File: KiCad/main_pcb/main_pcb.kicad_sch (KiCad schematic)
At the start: 14 parts, among them U5 TI TXB0104DR, U7 TI TXB0104DR, U8 CH340C

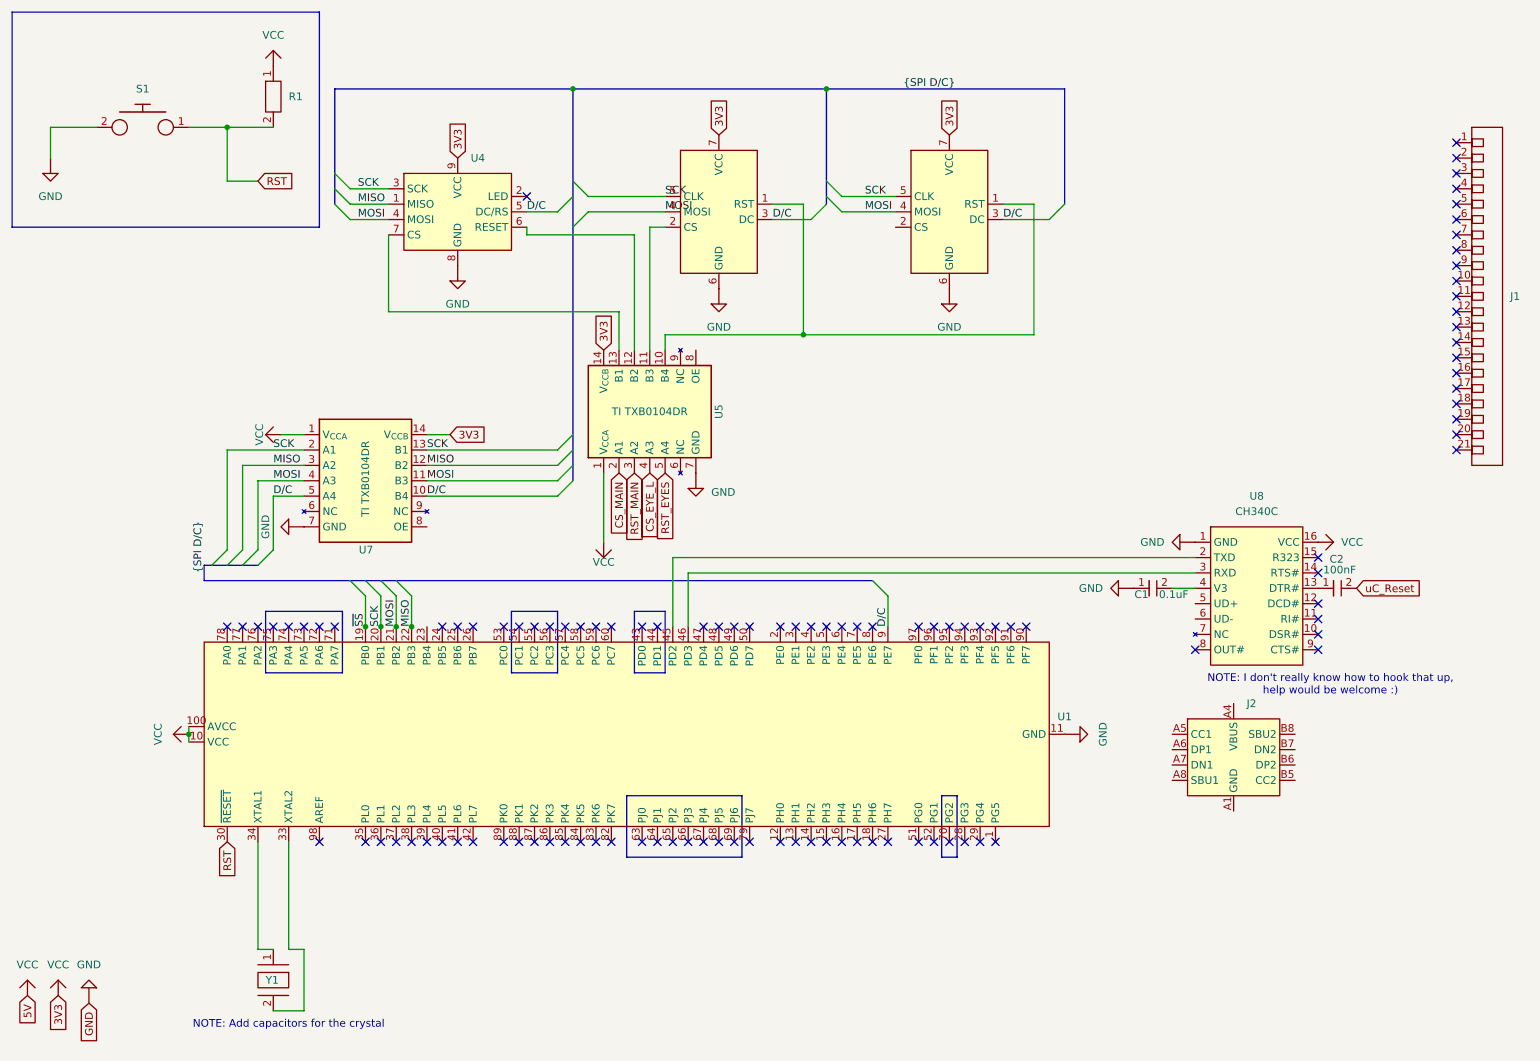
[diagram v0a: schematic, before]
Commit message: feat(KiCad): Enhances circuits, not done yet
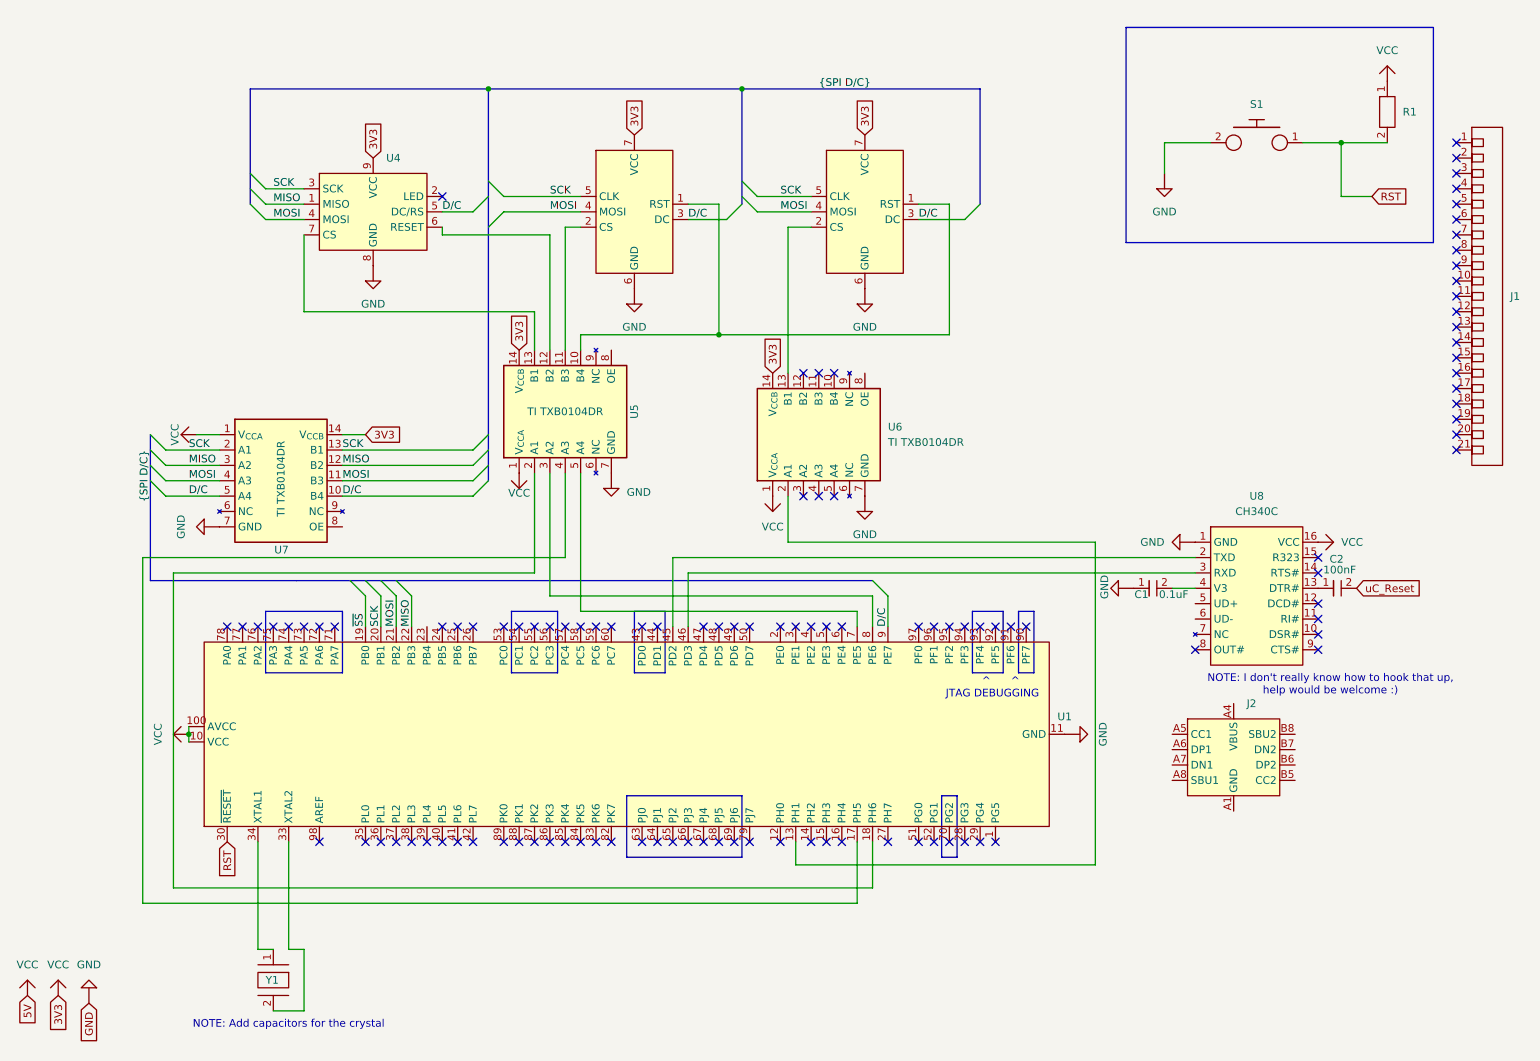
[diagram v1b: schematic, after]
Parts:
- added U6: TI TXB0104DR, symbol Lily's_Pad:TI TXB0104DR
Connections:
- net CS_EYE_L is gone; now on an unnamed net: U5.4 (A3)
- net CS_MAIN is gone; now on an unnamed net: U5.2 (A1)
- net RST_EYES is gone; now on an unnamed net: U5.5 (A4)
- net RST_MAIN is gone; now on an unnamed net: U5.3 (A2)
- net GND: now also U6.7 (GND)
- net VCC: now also U6.1 (V_{CCA}), U6.14 (V_{CCB})
- net at U2.2 (CS): now also U6.13 (B1)
- net at U1.13 (PH1): now also U6.2 (A1)
- no-connect marks 108 -> 109
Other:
- note added: "^ ^ JTAG DEBUGGING"
- moved on the sheet: R1, S1, U4, U5, U7

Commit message: feat(KiCad): Enhances circuits, not done yet
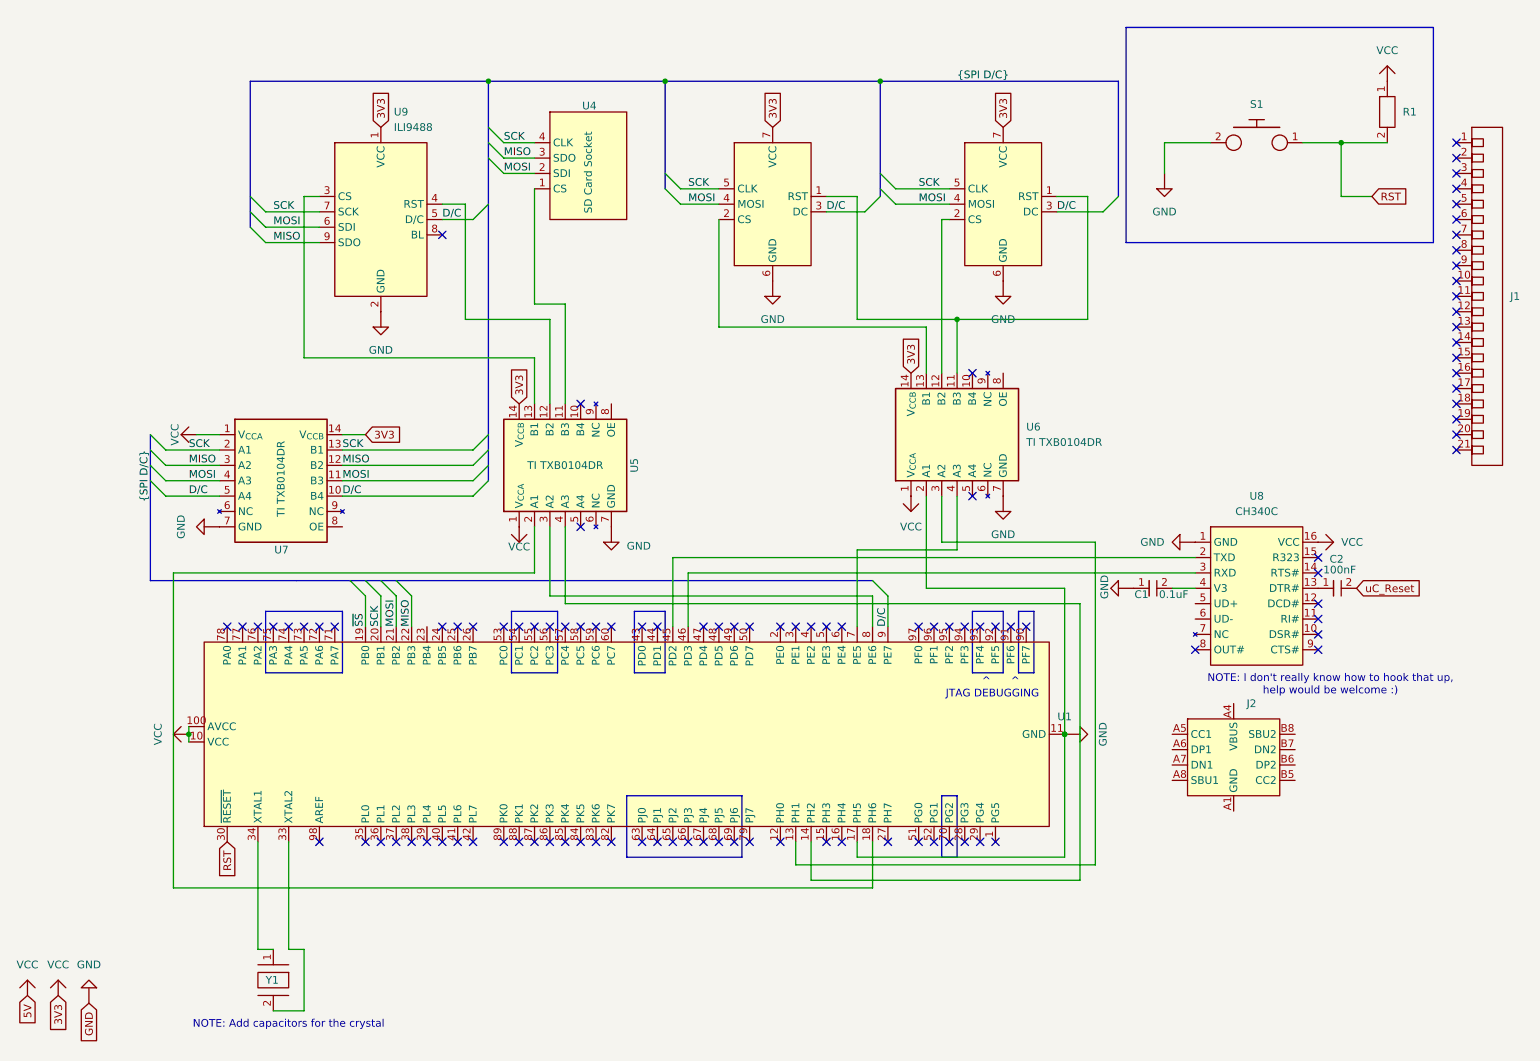
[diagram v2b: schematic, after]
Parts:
- removed U4: (no value), symbol Lily's_Pad:Main_LCD_?
- added U4: SD Card Socket, symbol Lily's_Pad:SD_Card_Socket
- added U9: ILI9488, symbol Lily's_Pad:ILI9488
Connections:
- net D/C: now also U9.5 (D/C)
- net GND: now also U1.17 (PH5), U6.2 (A1), U9.2 (GND)
- net MISO: now also U4.3 (SDO), U9.9 (SDO); no longer U1.22 (PB3)
- net MOSI: now also U4.2 (SDI), U9.6 (SDI); no longer U1.21 (PB2)
- net SCK: now also U4.4 (CLK), U9.7 (SCK); no longer U1.20 (PB1)
- net VCC: now also U9.1 (VCC)
- net ~{SS}: no longer U1.19 (PB0)
- net at U2.1 (RST), U3.1 (RST): now also U6.11 (B3); no longer U5.10 (B4)
- net at U2.2 (CS): now also U6.12 (B2); no longer U6.13 (B1)
- net at U3.2 (CS): now also U6.13 (B1); no longer U5.11 (B3)
- net at U5.12 (B2): now also U9.4 (RST)
- net at U5.13 (B1): now also U9.3 (CS)
- net at U5.4 (A3): now also U1.14 (PH2); no longer U1.17 (PH5)
- net at U5.5 (A4): no longer U1.7 (PE5)
- net at U1.13 (PH1): now also U6.3 (A2); no longer U6.2 (A1)
- net at U6.4 (A3): now also U1.7 (PE5)
- new net: U4.1 (CS), U5.11 (B3)
- no-connect marks 109 -> 106
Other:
- moved on the sheet: U5, U6
